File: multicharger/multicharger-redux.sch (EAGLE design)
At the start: 32 parts, among them J2 USB-A-SMD-KEYSTONE-931, J3 HEADER-8POS-, P1 TEST-POINT-1MM, P2 TEST-POINT-1MM, P3 TEST-POINT-1MM, P4 TEST-POINT-1MM, P5 TEST-POINT-1MM, P6 TEST-POINT-1MM, P7 1K, P8 TEST-POINT-1MM, P9 TEST-POINT-1MM, U1 MCP73831T-2ACI/OT, U2 MCP73831T-2ACI/OT, U3 MCP73831T-2ACI/OT, U4 MCP73831T-2ACI/OT

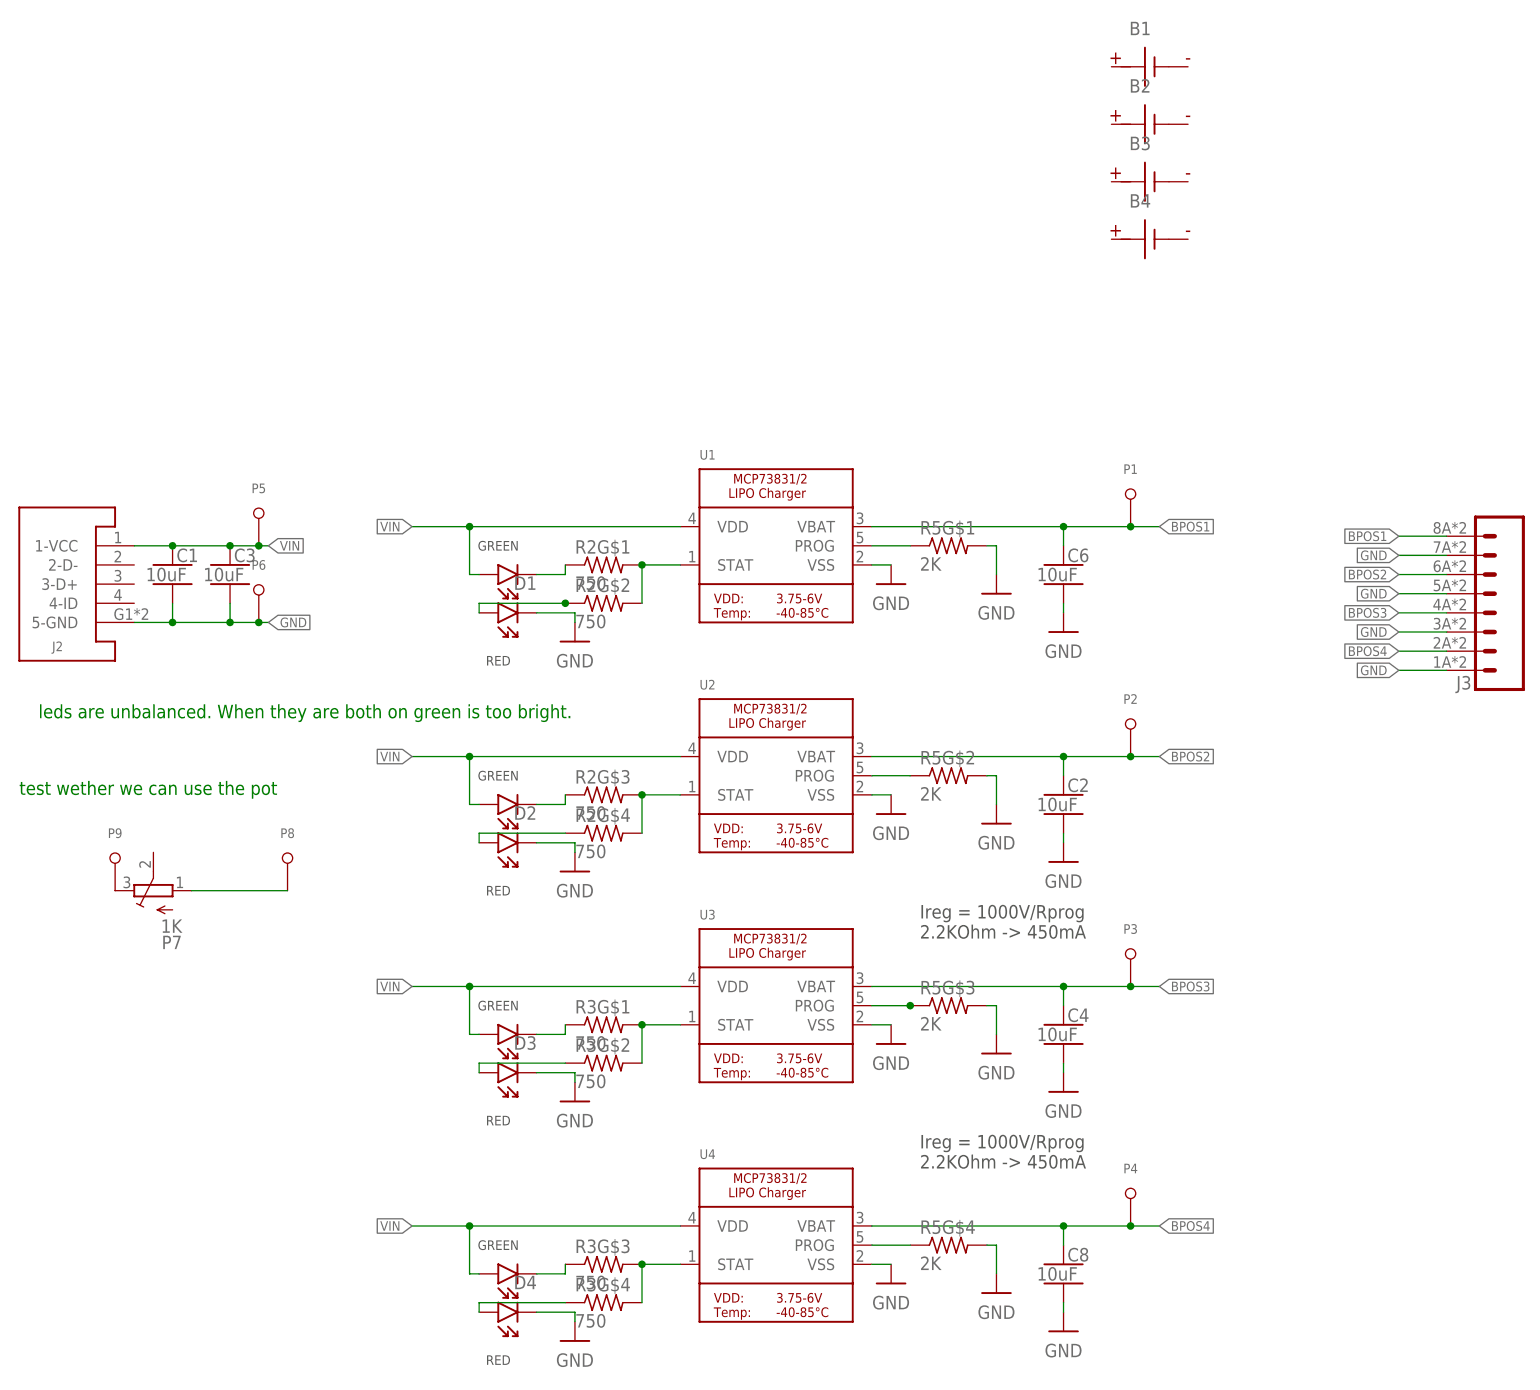
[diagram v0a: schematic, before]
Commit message: simplified charging board
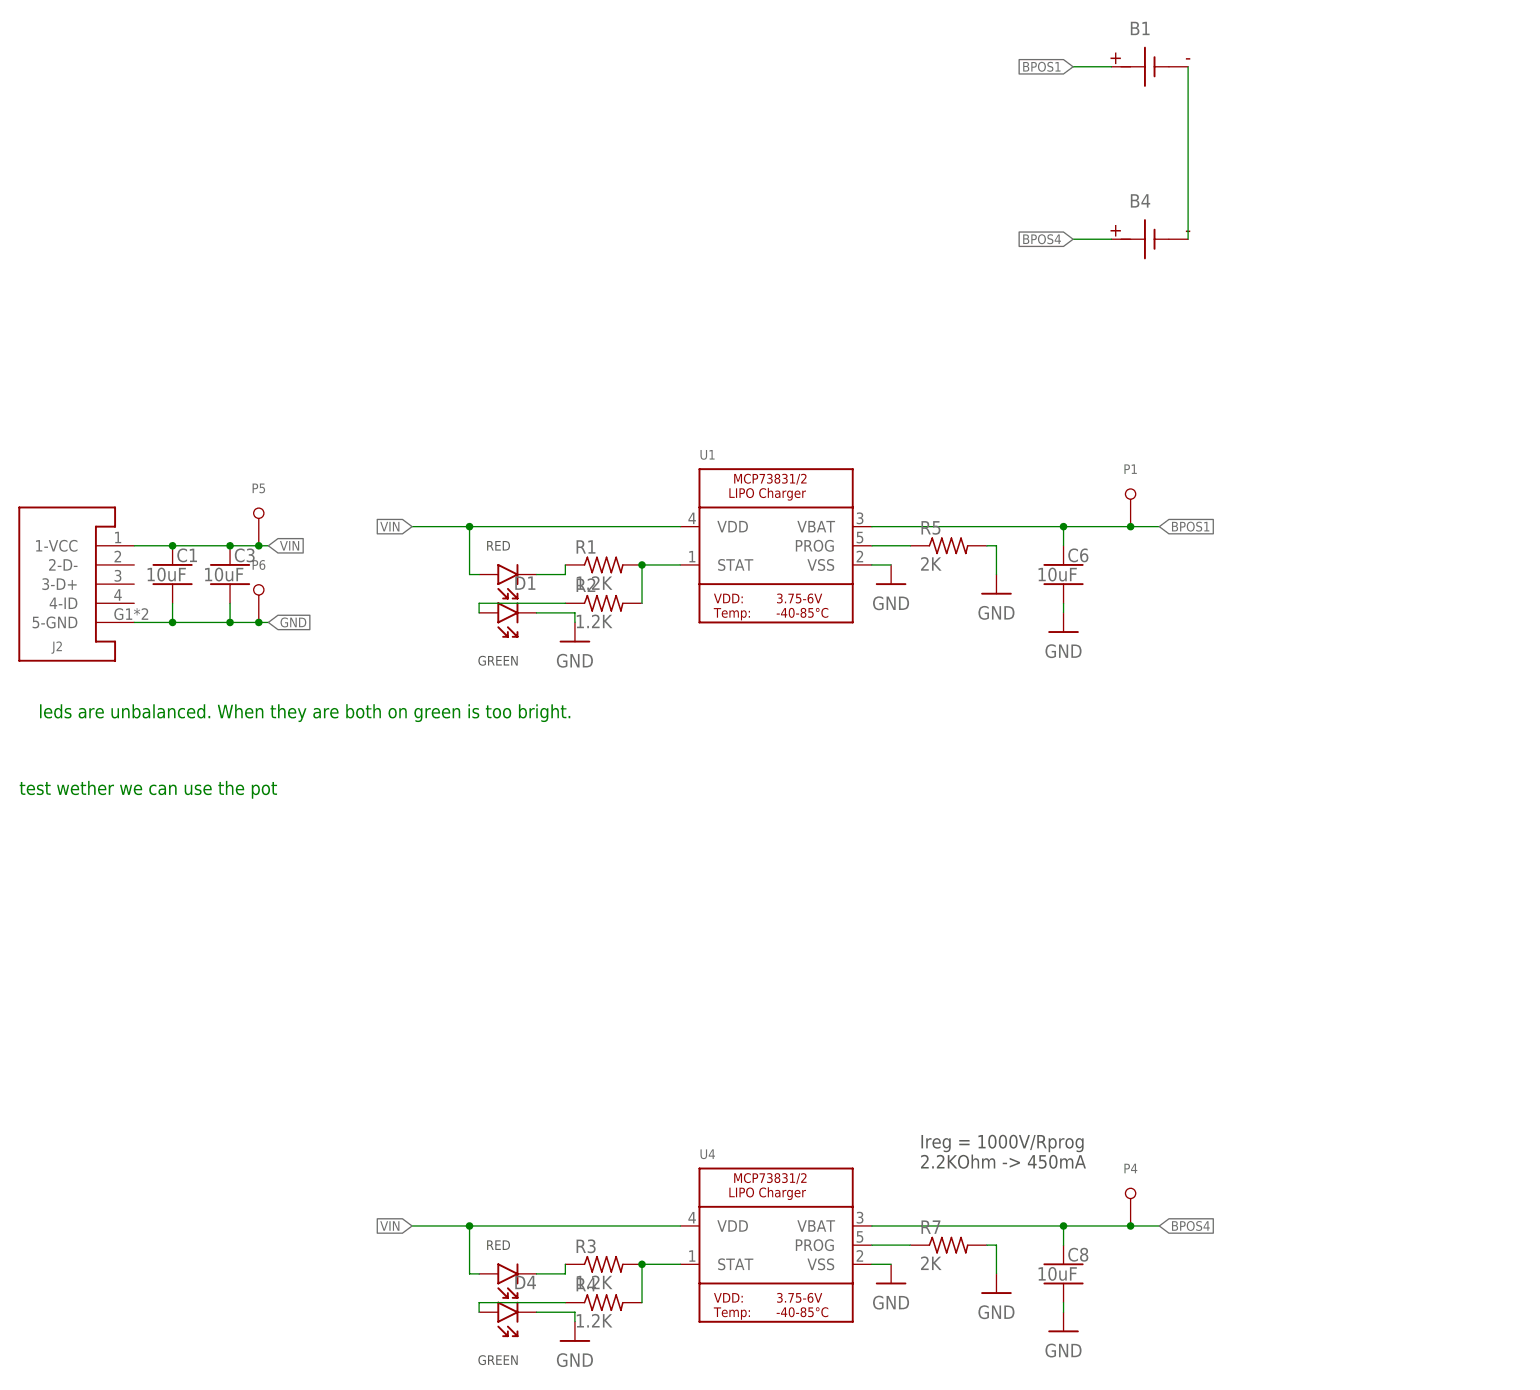
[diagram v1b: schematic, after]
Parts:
- removed B2, B3: BATTERY-SMD, quadparts_prebuilt:BATTERY-SMD
- removed C2, C4: 10uF, quadparts_prebuilt:CAPACITOR-NP_SMD-0603_CERAMIC-10UF
- removed D2, D3: LED-2X-GREEN/RED-1.6X1.5MM, RemoteParts:LED-2X-GREEN/RED-1.6X1.5MM
- removed J3: HEADER-8POS-, quadparts_prebuilt:HEADER-8POS-
- removed P2, P3, P8, P9: TEST-POINT-1MM, RemoteParts:TEST-POINT-1MM
- removed P7: 1K, RemoteParts:TRIMPOT-BOT-ADJUST-1K
- removed U2, U3: MCP73831T-2ACI/OT, RemoteParts:MCP73831/2
- added R1, R4: 1.2K, quadparts_prebuilt:RESISTOR_SMD-2012-0805-1.2K
- added R7: 2K, quadparts_prebuilt:RESISTOR_SMD-2012-0805-2K
- C1, C3, C6, C8: device quadparts_prebuilt:CAPACITOR-NP_SMD-0603_CERAMIC-10UF -> quadparts_prebuilt:CAPACITOR-NP_SMD-2012-0805_CERAMIC-10UF
- R2, R3: value 750 -> 1.2K; device quadparts_prebuilt:RESISTOR-PACK-4X-750 -> quadparts_prebuilt:RESISTOR_SMD-2012-0805-1.2K
- R5: device quadparts_prebuilt:RESISTOR-PACK-4X-2K -> quadparts_prebuilt:RESISTOR_SMD-2012-0805-2K
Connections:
- removed net BPOS2: C2.1, J3.6, P2.T, U2.VBAT
- removed net BPOS3: C4.1, J3.4, P3.T, U3.VBAT
- removed net N$10: D3.C2, R3G$1.1
- removed net N$17: P7.A, P8.T
- removed net N$18: P7.E, P9.T
- removed net N$3: R2G$3.2, R2G$4.2, U2.STAT
- removed net N$4: R5G$2.1, U2.PROG
- removed net N$5: D2.A1, R2G$4.1
- removed net N$6: D2.C2, R2G$3.1
- removed net N$7: R3G$1.2, R3G$2.2, U3.STAT
- removed net N$8: R5G$3.1, U3.PROG
- removed net N$9: D3.A1, R3G$2.1
- net BPOS1: now also B1.P; no longer J3.8
- net BPOS4: now also B4.P; no longer J3.2
- net GND: now also B1.N, B4.N, R5.2, R7.2; no longer C2.2, C4.2, D2.C1, D3.C1, J3.1, J3.3, J3.5, J3.7, R5G$1.2, R5G$2.2, R5G$3.2, R5G$4.2, U2.VSS, U3.VSS
- net N$1: now also R2.1; no longer R2G$2.1
- net N$11: now also R1.2, R2.2; no longer R2G$1.2, R2G$2.2
- net N$12: now also R5.1; no longer R5G$1.1
- net N$13: now also R3.2, R4.2; no longer R3G$3.2, R3G$4.2
- net N$14: now also R7.1; no longer R5G$4.1
- net N$15: now also R4.1; no longer R3G$4.1
- net N$16: now also R3.1; no longer R3G$3.1
- net N$2: now also R1.1; no longer R2G$1.1
- net VIN: no longer D2.A2, D3.A2, U2.VDD, U3.VDD
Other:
- moved on the sheet: R2, R3

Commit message: bump rc
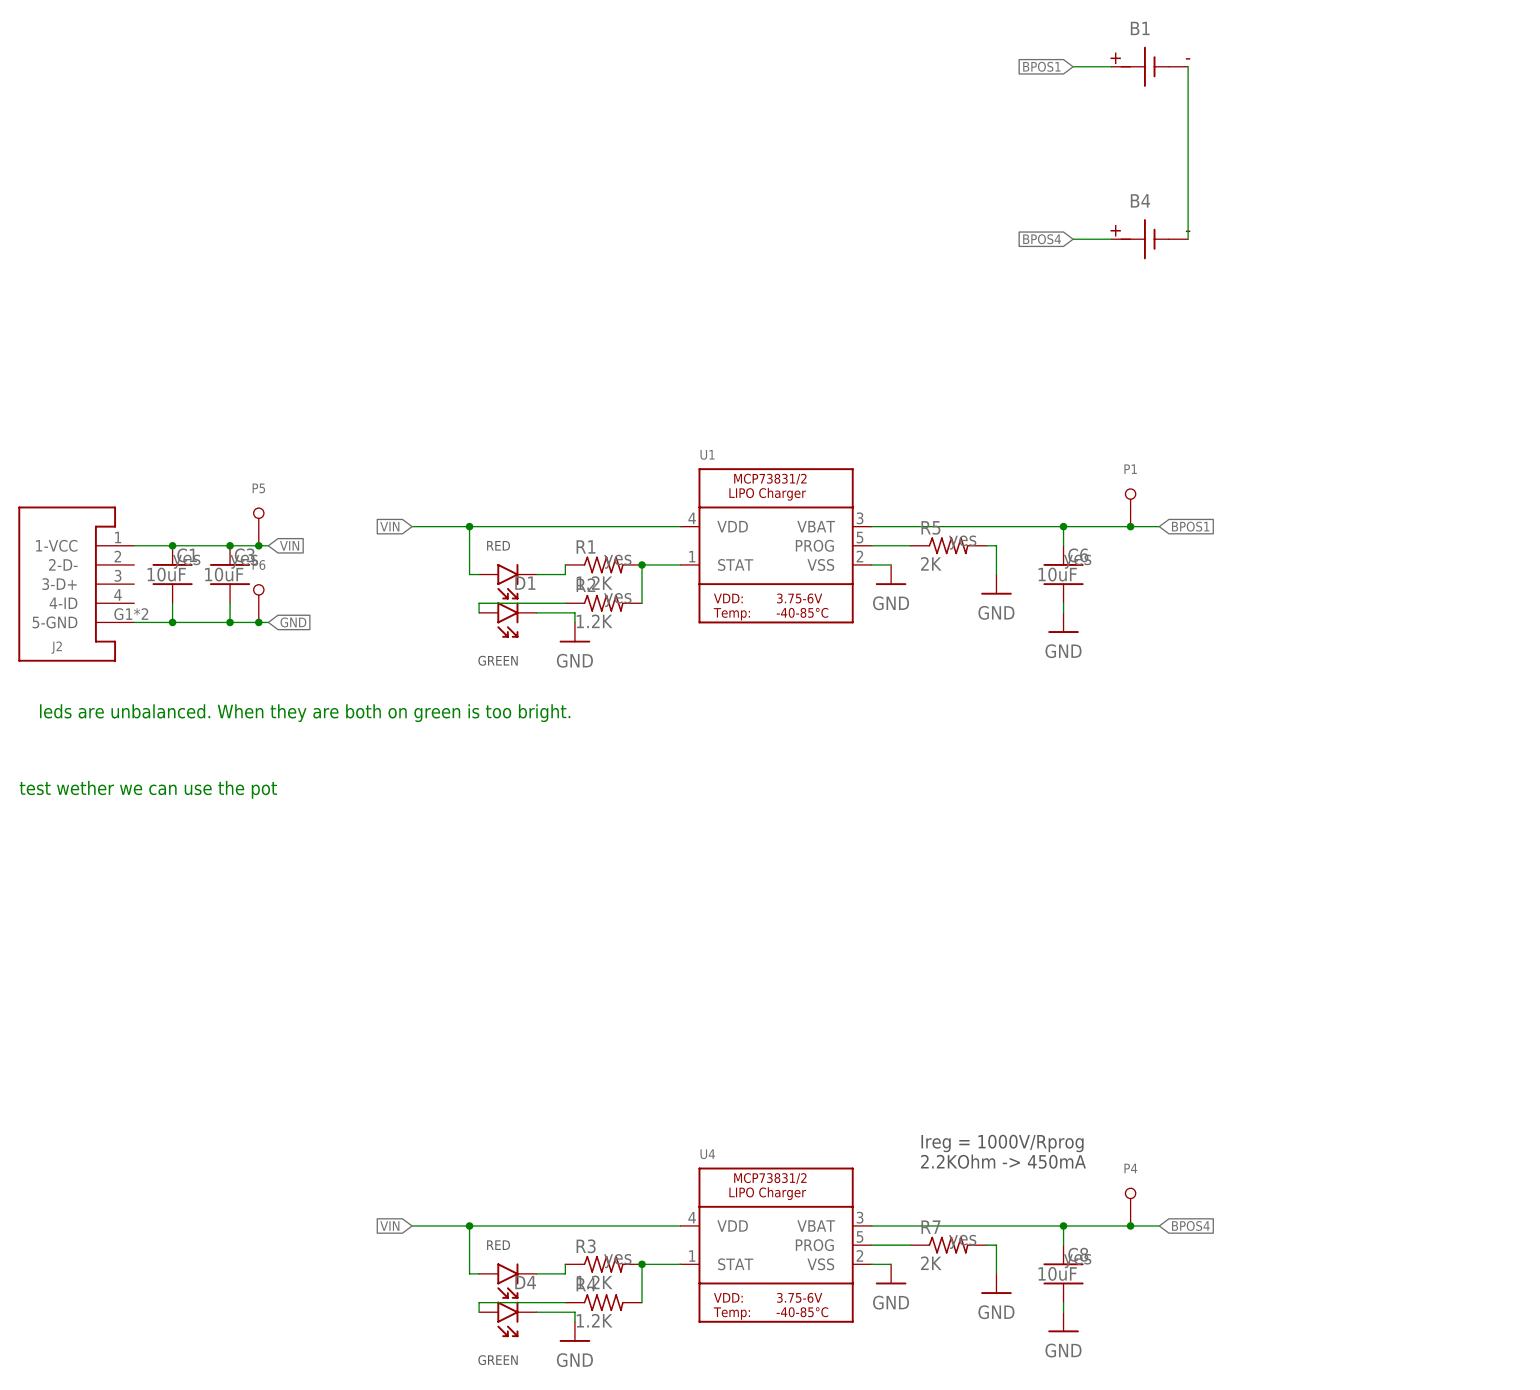
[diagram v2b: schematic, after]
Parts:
- C1, C3, C6, C8, R1, R2, R3, R5, R7: SUBSTITUTE_OK (none) -> yes
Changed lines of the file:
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@@
 <?xml version="1.0" encoding="utf-8"?>
 <!DOCTYPE eagle SYSTEM "eagle.dtd">
-<eagle version="9.4.0">
+<eagle version="9.6.2">
 <drawing>
 <settings>
@@
 <setting verticaltext="up"/>
 </settings>
-<grid distance="0.05" unitdist="inch" unit="inch" style="lines" multiple="1" display="no" altdistance="0.01" altunitdist="inch" altunit="inch"/>
+<grid distance="0.1" unitdist="inch" unit="inch" style="lines" multiple="1" display="no" altdistance="0.01" altunitdist="inch" altunit="inch"/>
 <layers>
 <layer number="1" name="Top" color="4" fill="1" visible="no" active="no"/>
@@
 <part name="P+22" library="quadparts_prebuilt" deviceset="GND" device=""/>
 <part name="P+21" library="quadparts_prebuilt" deviceset="GND" device=""/>
-<part name="C6" library="quadparts_prebuilt" deviceset="CAPACITOR-NP_" device="SMD-2012-0805_CERAMIC-10UF" value="10uF"/>
+<part name="C6" library="quadparts_prebuilt" deviceset="CAPACITOR-NP_" device="SMD-2012-0805_CERAMIC-10UF" value="10uF">
+<attribute name="SUBSTITUTE_OK" value="yes"/>
+</part>
 <part name="P+23" library="quadparts_prebuilt" deviceset="GND" device=""/>
 <part name="D1" library="RemoteParts" deviceset="LED-2X" device="-GREEN/RED-1.6X1.5MM" value="LED-2X-GREEN/RED-1.6X1.5MM"/>
@@
 <part name="P+13" library="quadparts_prebuilt" deviceset="GND" device=""/>
 <part name="P+14" library="quadparts_prebuilt" deviceset="GND" device=""/>
-<part name="C8" library="quadparts_prebuilt" deviceset="CAPACITOR-NP_" device="SMD-2012-0805_CERAMIC-10UF" value="10uF"/>
+<part name="C8" library="quadparts_prebuilt" deviceset="CAPACITOR-NP_" device="SMD-2012-0805_CERAMIC-10UF" value="10uF">
+<attribute name="SUBSTITUTE_OK" value="yes"/>
+</part>
 <part name="P+15" library="quadparts_prebuilt" deviceset="GND" device=""/>
 <part name="D4" library="RemoteParts" deviceset="LED-2X" device="-GREEN/RED-1.6X1.5MM" value="LED-2X-GREEN/RED-1.6X1.5MM"/>
@@
 <part name="P5" library="RemoteParts" deviceset="TEST-POINT" device="-1MM" value="TEST-POINT-1MM"/>
 <part name="P6" library="RemoteParts" deviceset="TEST-POINT" device="-1MM" value="TEST-POINT-1MM"/>
-<part name="C1" library="quadparts_prebuilt" deviceset="CAPACITOR-NP_" device="SMD-2012-0805_CERAMIC-10UF" value="10uF"/>
-<part name="C3" library="quadparts_prebuilt" deviceset="CAPACITOR-NP_" device="SMD-2012-0805_CERAMIC-10UF" value="10uF"/>
+<part name="C1" library="quadparts_prebuilt" deviceset="CAPACITOR-NP_" device="SMD-2012-0805_CERAMIC-10UF" value="10uF">
+<attribute name="SUBSTITUTE_OK" value="yes"/>
+</part>
+<part name="C3" library="quadparts_prebuilt" deviceset="CAPACITOR-NP_" device="SMD-2012-0805_CERAMIC-10UF" value="10uF">
+<attribute name="SUBSTITUTE_OK" value="yes"/>
+</part>
 <part name="B1" library="quadparts_prebuilt" deviceset="BATTERY" device="-SMD"/>
 <part name="B4" library="quadparts_prebuilt" deviceset="BATTERY" device="-SMD"/>
-<part name="R1" library="quadparts_prebuilt" deviceset="RESISTOR_" device="SMD-2012-0805-1.2K" value="1.2K"/>
-<part name="R2" library="quadparts_prebuilt" deviceset="RESISTOR_" device="SMD-2012-0805-1.2K" value="1.2K"/>
-<part name="R3" library="quadparts_prebuilt" deviceset="RESISTOR_" device="SMD-2012-0805-1.2K" value="1.2K"/>
+<part name="R1" library="quadparts_prebuilt" deviceset="RESISTOR_" device="SMD-2012-0805-1.2K" value="1.2K">
+<attribute name="SUBSTITUTE_OK" value="yes"/>
+</part>
+<part name="R2" library="quadparts_prebuilt" deviceset="RESISTOR_" device="SMD-2012-0805-1.2K" value="1.2K">
+<attribute name="SUBSTITUTE_OK" value="yes"/>
+</part>
+<part name="R3" library="quadparts_prebuilt" deviceset="RESISTOR_" device="SMD-2012-0805-1.2K" value="1.2K">
+<attribute name="SUBSTITUTE_OK" value="yes"/>
+</part>
 <part name="R4" library="quadparts_prebuilt" deviceset="RESISTOR_" device="SMD-2012-0805-1.2K" value="1.2K"/>
-<part name="R5" library="quadparts_prebuilt" deviceset="RESISTOR_" device="SMD-2012-0805-2K" value="2K"/>
-<part name="R7" library="quadparts_prebuilt" deviceset="RESISTOR_" device="SMD-2012-0805-2K" value="2K"/>
+<part name="R5" library="quadparts_prebuilt" deviceset="RESISTOR_" device="SMD-2012-0805-2K" value="2K">
+<attribute name="SUBSTITUTE_OK" value="yes"/>
+</part>
+<part name="R7" library="quadparts_prebuilt" deviceset="RESISTOR_" device="SMD-2012-0805-2K" value="2K">
+<attribute name="SUBSTITUTE_OK" value="yes"/>
+</part>
 </parts>
 <sheets>
@@
 <attribute name="VALUE" x="231.394" y="180.721" size="1.778" layer="96"/>
 <attribute name="NAME" x="235.458" y="183.261" size="1.778" layer="95"/>
+<attribute name="SUBSTITUTE_OK" x="234.95" y="182.88" size="1.778" layer="96"/>
 </instance>
 <instance part="P+23" gate="1" x="226.06" y="179.07" smashed="yes">
@@
 <attribute name="VALUE" x="231.394" y="88.011" size="1.778" layer="96"/>
 <attribute name="NAME" x="235.458" y="90.551" size="1.778" layer="95"/>
+<attribute name="SUBSTITUTE_OK" x="234.95" y="90.17" size="1.778" layer="96"/>
 </instance>
 <instance part="P+15" gate="1" x="226.06" y="86.36" smashed="yes">
@@
 <attribute name="VALUE" x="113.284" y="180.721" size="1.778" layer="96"/>
 <attribute name="NAME" x="117.348" y="183.261" size="1.778" layer="95"/>
+<attribute name="SUBSTITUTE_OK" x="116.84" y="182.88" size="1.778" layer="96"/>
 </instance>
 <instance part="C3" gate="G$1" x="124.46" y="182.88" smashed="yes">
 <attribute name="VALUE" x="120.904" y="180.721" size="1.778" layer="96"/>
 <attribute name="NAME" x="124.968" y="183.261" size="1.778" layer="95"/>
+<attribute name="SUBSTITUTE_OK" x="124.46" y="182.88" size="1.778" layer="96"/>
 </instance>
 <instance part="B1" gate="G$1" x="246.38" y="248.92" smashed="yes">
@@
 <attribute name="VALUE" x="170.18" y="179.578" size="1.778" layer="96"/>
 <attribute name="NAME" x="170.18" y="184.3786" size="1.778" layer="95"/>
+<attribute name="SUBSTITUTE_OK" x="173.99" y="182.88" size="1.778" layer="96"/>
 </instance>
 <instance part="R2" gate="G$1" x="173.99" y="177.8" smashed="yes">
 <attribute name="VALUE" x="170.18" y="174.498" size="1.778" layer="96"/>
 <attribute name="NAME" x="170.18" y="179.2986" size="1.778" layer="95"/>
+<attribute name="SUBSTITUTE_OK" x="173.99" y="177.8" size="1.778" layer="96"/>
 </instance>
 <instance part="R3" gate="G$1" x="173.99" y="90.17" smashed="yes">
 <attribute name="VALUE" x="170.18" y="86.868" size="1.778" layer="96"/>
 <attribute name="NAME" x="170.18" y="91.6686" size="1.778" layer="95"/>
+<attribute name="SUBSTITUTE_OK" x="173.99" y="90.17" size="1.778" layer="96"/>
 </instance>
 <instance part="R4" gate="G$1" x="173.99" y="85.09" smashed="yes">
@@
 <attribute name="VALUE" x="215.9" y="182.118" size="1.778" layer="96"/>
 <attribute name="NAME" x="215.9" y="186.9186" size="1.778" layer="95"/>
+<attribute name="SUBSTITUTE_OK" x="219.71" y="185.42" size="1.778" layer="96"/>
 </instance>
 <instance part="R7" gate="G$1" x="219.71" y="92.71" smashed="yes">
 <attribute name="VALUE" x="215.9" y="89.408" size="1.778" layer="96"/>
 <attribute name="NAME" x="215.9" y="94.2086" size="1.778" layer="95"/>
+<attribute name="SUBSTITUTE_OK" x="219.71" y="92.71" size="1.778" layer="96"/>
 </instance>
 </instances>
